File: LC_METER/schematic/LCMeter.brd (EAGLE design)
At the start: 70 x 125 mm, 212 parts, among them IC1 MEGA8535, IC10 MC34063, IC2 74HC595, IC3 74HC595, IC4 74HC595, IC5 74HC595, IC6 74HC595, IC7 LM324, IC8 7905, IC9 LM317, J10 0, J100 0, J11 0, J4 0, J6 0, J8 0, Q1 12MHz, T1 BC847, T2 BC857, T3 BC847, T4 BC847, T5 BC847, T6 BC847, T7 BC857, X1 MCU_PROGRAMMING, X2 L_X, X3 C_X, X4 USB_MICRO, X5 USB_B

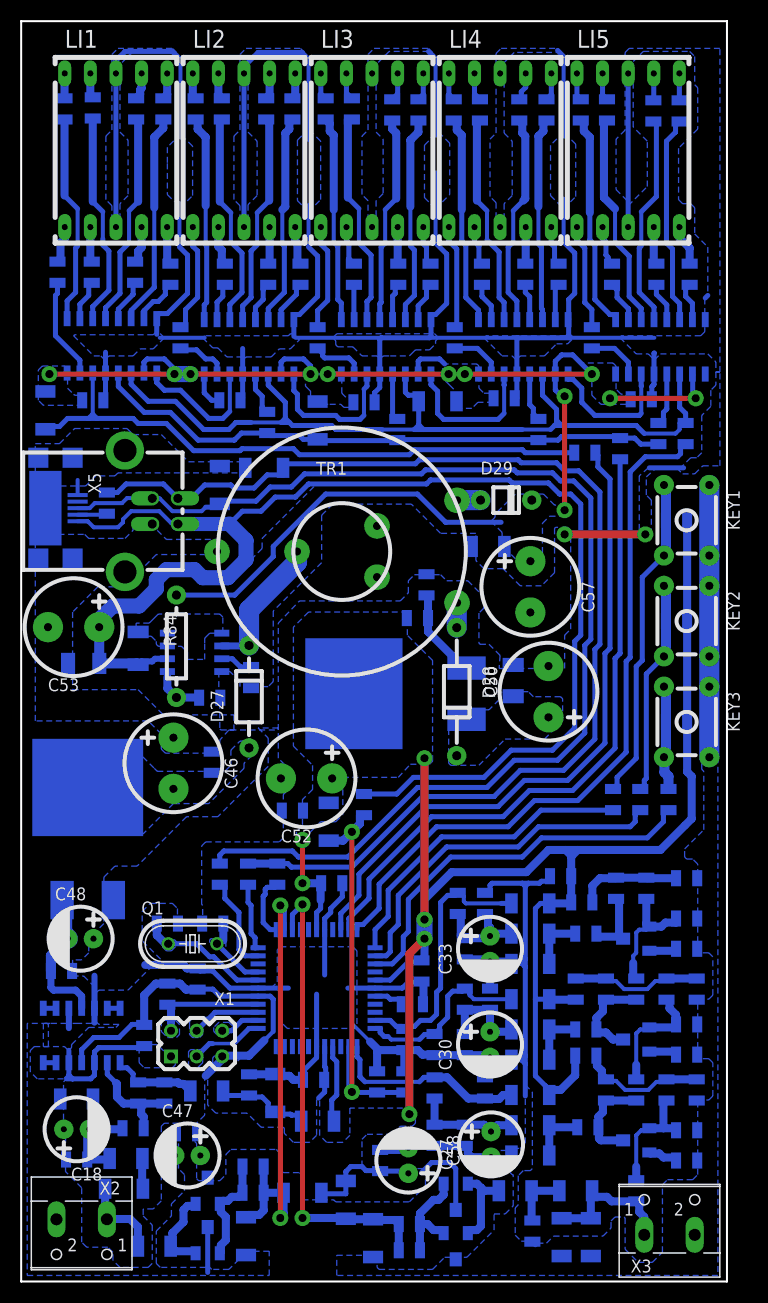
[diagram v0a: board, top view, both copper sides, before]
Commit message: LCMeter Route finished
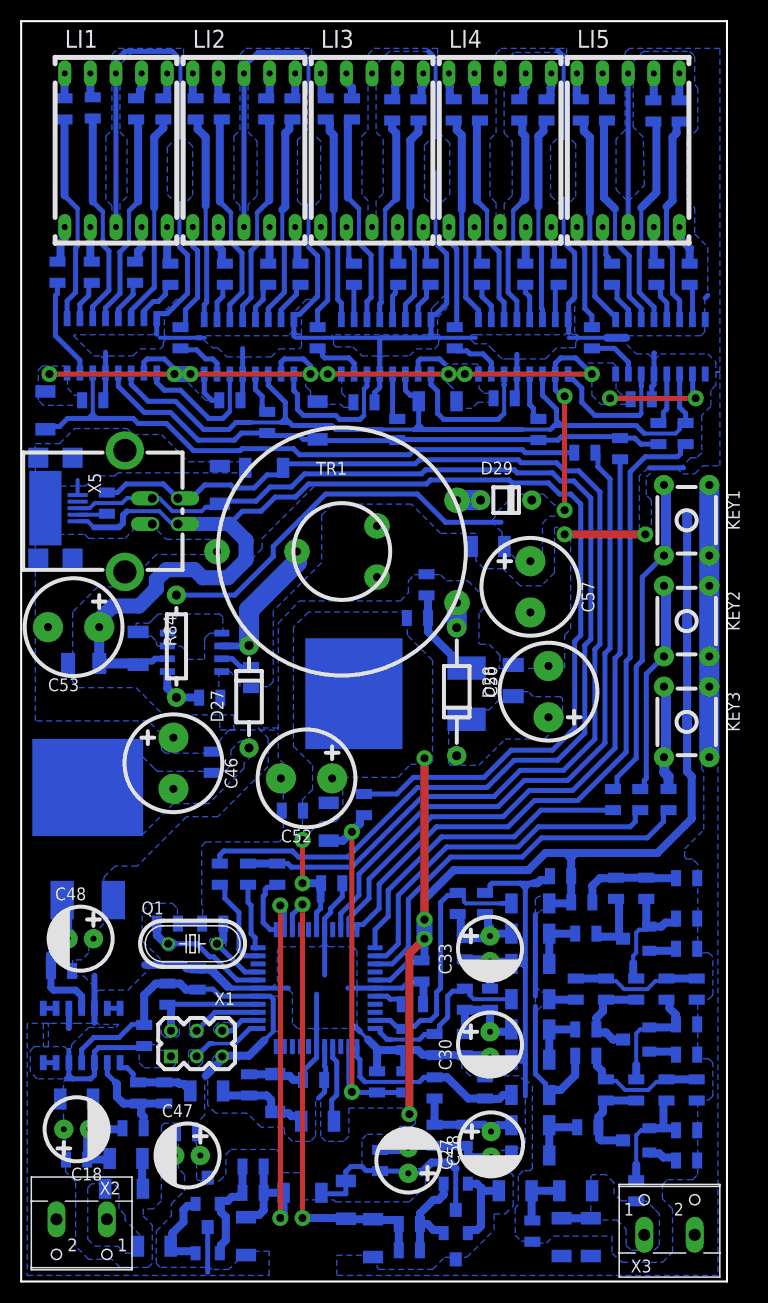
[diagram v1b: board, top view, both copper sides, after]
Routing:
- net GND: track 423.1 -> 406.6 mm
- net N$114: track 13.9 -> 2.90 mm
- net N$12: track 8.44 -> 0.00 mm
- net +5V_FINE: track 217.7 -> 212.7 mm
- net VCC_ROUGH: track 143.3 -> 141.6 mm
- net L_ADC: track 10.0 -> 9.45 mm
- added copper zone on layer 16, net N$114
- added copper zone on layer 16, net N$12

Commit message: LC meter schematic. Power stabilizer values fix
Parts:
- R81: value 5K1 -> 1K0
- R82: value 1K7 -> 3K0
- R84: value 5K1 -> 4K7
- R85: value 1K7 -> 1K6
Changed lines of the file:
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@@
 <grid distance="0.1" unitdist="mm" unit="mm" style="lines" multiple="1" display="yes" altdistance="0.025" altunitdist="inch" altunit="inch"/>
 <layers>
-<layer number="1" name="Top" color="4" fill="1" visible="no" active="yes"/>
+<layer number="1" name="Top" color="4" fill="1" visible="yes" active="yes"/>
 <layer number="2" name="Route2" color="1" fill="3" visible="no" active="no"/>
 <layer number="3" name="Route3" color="4" fill="3" visible="no" active="no"/>
@@
 <layer number="21" name="tPlace" color="7" fill="1" visible="yes" active="yes"/>
 <layer number="22" name="bPlace" color="7" fill="1" visible="yes" active="yes"/>
-<layer number="23" name="tOrigins" color="15" fill="1" visible="no" active="yes"/>
-<layer number="24" name="bOrigins" color="15" fill="1" visible="no" active="yes"/>
+<layer number="23" name="tOrigins" color="15" fill="1" visible="yes" active="yes"/>
+<layer number="24" name="bOrigins" color="15" fill="1" visible="yes" active="yes"/>
 <layer number="25" name="tNames" color="7" fill="1" visible="no" active="yes"/>
 <layer number="26" name="bNames" color="7" fill="1" visible="no" active="yes"/>
@@
 <element name="C56" library="__MyCommonLib1" package="RSMD_1206_BIG_GAP" value="0.47uFx16V" x="46.3" y="72.9" rot="MR180"/>
 <element name="C57" library="__MyCommonLib1" package="CE_10MM" value="470uFx16V" x="50.5" y="68.9" rot="R90"/>
-<element name="R84" library="__MyCommonLib1" package="R0207" value="5K1" x="15.4" y="63" rot="R90"/>
-<element name="R85" library="__MyCommonLib1" package="RSMD_0805" value="1K7" x="18.7" y="57.9" rot="MR0"/>
+<element name="R84" library="__MyCommonLib1" package="R0207" value="4K7" x="15.4" y="63" rot="R90"/>
+<element name="R85" library="__MyCommonLib1" package="RSMD_0805" value="1K6" x="18.7" y="57.9" rot="MR0"/>
 <element name="C49" library="__MyCommonLib1" package="RSMD_1206" value="0.47uFx16V" x="48.8" y="59.6" rot="MR270"/>
 <element name="C50" library="__MyCommonLib1" package="CE_10MM" value="470uFx16V" x="52.3" y="58.5" rot="R270"/>
@@
 <element name="C51" library="__MyCommonLib1" package="RSMD_0805" value="0.47uFx16V" x="26.9" y="46.7" rot="MR180"/>
 <element name="C52" library="__MyCommonLib1" package="CE_10MM" value="47uFx16V" x="28.3" y="49.9"/>
-<element name="R81" library="__MyCommonLib1" package="RSMD_0805" value="5K1" x="39.3" y="65.8" rot="MR180"/>
-<element name="R82" library="__MyCommonLib1" package="RSMD_0805" value="1K7" x="40.2" y="69.1" rot="MR270"/>
+<element name="R81" library="__MyCommonLib1" package="RSMD_0805" value="1K0" x="39.3" y="65.8" rot="MR180"/>
+<element name="R82" library="__MyCommonLib1" package="RSMD_0805" value="3K0" x="40.2" y="69.1" rot="MR270"/>
 <element name="IC8" library="__MyCommonLib1" package="D2PAK" value="7905" x="6.6" y="49" rot="MR0"/>
 <element name="C3" library="__MyCommonLib1" package="RSMD_0805" value="0.1uF" x="38.8" y="27.5" rot="MR0"/>

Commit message: LC Meter change some values
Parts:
- C47, C58: value 4.7uF -> 100uFx10V
- R54, R67, R69, R71: value 100K -> 120K
- R55, R74: value 4K7 -> 2K2
- R58: value 20K -> 24K
- R59: value 300R -> 1K0
- R75, R77, R79: value 25K -> 24K
- R86, R87, R88: value 1K0 -> 10K
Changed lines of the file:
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@@
 <layer number="49" name="Reference" color="7" fill="1" visible="no" active="yes"/>
 <layer number="51" name="tDocu" color="7" fill="1" visible="no" active="yes"/>
-<layer number="52" name="bDocu" color="7" fill="1" visible="no" active="yes"/>
+<layer number="52" name="bDocu" color="7" fill="1" visible="yes" active="yes"/>
 <layer number="91" name="Nets" color="2" fill="1" visible="no" active="no"/>
 <layer number="92" name="Busses" color="1" fill="1" visible="no" active="no"/>
@@
 <element name="R8" library="__MyCommonLib1" package="RSMD_0805" value="68R" x="25.4" y="40.4" rot="MR270"/>
 <element name="R9" library="__MyCommonLib1" package="RSMD_0805" value="1K5" x="22.5" y="40.4" rot="MR270"/>
-<element name="R55" library="__MyCommonLib1" package="RSMD_0805" value="4K7" x="23" y="11.4" rot="MR0"/>
+<element name="R55" library="__MyCommonLib1" package="RSMD_0805" value="2K2" x="23" y="11.4" rot="MR0"/>
 <element name="C17" library="__MyCommonLib1" package="RSMD_0805" value="1nF" x="23" y="8.8" rot="MR180"/>
 <element name="T1" library="__MyCommonLib1" package="SOT23_SMALL_PADS" value="BC847" x="18.5" y="9" rot="MR180"/>
@@
 <element name="C19" library="__MyCommonLib1" package="RSMD_1206_BIG_GAP" value="0.47uF" x="5.5" y="18.1" rot="MR180"/>
 <element name="R60" library="__MyCommonLib1" package="RSMD_0805" value="4K7" x="5.5" y="12.1" rot="MR0"/>
-<element name="R58" library="__MyCommonLib1" package="RSMD_0805" value="20K" x="11.1" y="15.2" rot="MR180"/>
+<element name="R58" library="__MyCommonLib1" package="RSMD_0805" value="24K" x="11.1" y="15.2" rot="MR180"/>
 <element name="C16" library="__MyCommonLib1" package="RSMD_0805" value="0.1uF" x="14.2" y="18.7" rot="MR270"/>
 <element name="IC7" library="__MyCommonLib1" package="SOIC14" value="LM324" x="6" y="24.4" rot="MR90"/>
 <element name="C25" library="__MyCommonLib1" package="RSMD_0805" value="0.1uF" x="4" y="30.8" rot="MR180"/>
 <element name="C21" library="__MyCommonLib1" package="RSMD_0805" value="0.1uF" x="12.2" y="24.4" rot="MR90"/>
-<element name="R54" library="__MyCommonLib1" package="RSMD_0805" value="100K" x="11.6" y="18.7" rot="MR90"/>
-<element name="R59" library="__MyCommonLib1" package="RSMD_1206_BIG_GAP" value="300R" x="18.4" y="18.9" rot="MR180"/>
+<element name="R54" library="__MyCommonLib1" package="RSMD_0805" value="120K" x="11.6" y="18.7" rot="MR90"/>
+<element name="R59" library="__MyCommonLib1" package="RSMD_1206_BIG_GAP" value="1K0" x="18.4" y="18.9" rot="MR180"/>
 <element name="D10" library="__MyCommonLib1" package="SOD-80" value="LL4148" x="25.2" y="18.7" rot="MR90"/>
 <element name="C20" library="__MyCommonLib1" package="RSMD_0805" value="0.1uF" x="22.6" y="19.5" rot="MR90"/>
-<element name="R74" library="__MyCommonLib1" package="RSMD_0805" value="4K7" x="38.5" y="3.1" rot="MR180"/>
+<element name="R74" library="__MyCommonLib1" package="RSMD_0805" value="2K2" x="38.5" y="3.1" rot="MR180"/>
 <element name="C39" library="__MyCommonLib1" package="RSMD_0805" value="1nF" x="38.5" y="5.7" rot="MR0"/>
 <element name="T3" library="__MyCommonLib1" package="SOT23_SMALL_PADS" value="BC847" x="43.1" y="8.4" rot="MR0"/>
@@
 <element name="T4" library="__MyCommonLib1" package="SOT23_SMALL_PADS" value="BC847" x="61" y="14" rot="MR90"/>
 <element name="C41" library="__MyCommonLib1" package="RSMD_0805" value="0.1uF" x="61" y="9" rot="MR270"/>
-<element name="R75" library="__MyCommonLib1" package="RSMD_0805" value="25K" x="66" y="15" rot="MR0"/>
-<element name="R67" library="__MyCommonLib1" package="RSMD_0805" value="100K" x="64" y="19" rot="MR90"/>
+<element name="R75" library="__MyCommonLib1" package="RSMD_0805" value="24K" x="66" y="15" rot="MR0"/>
+<element name="R67" library="__MyCommonLib1" package="RSMD_0805" value="120K" x="64" y="19" rot="MR90"/>
 <element name="R68" library="__MyCommonLib1" package="RSMD_0805" value="1K0" x="58" y="19" rot="MR90"/>
 <element name="R76" library="__MyCommonLib1" package="RSMD_0805" value="100R" x="66" y="12" rot="MR0"/>
@@
 <element name="T5" library="__MyCommonLib1" package="SOT23_SMALL_PADS" value="BC847" x="61" y="24" rot="MR90"/>
 <element name="C42" library="__MyCommonLib1" package="RSMD_0805" value="0.1uF" x="61" y="19" rot="MR270"/>
-<element name="R77" library="__MyCommonLib1" package="RSMD_0805" value="25K" x="66" y="25.5" rot="MR0"/>
-<element name="R69" library="__MyCommonLib1" package="RSMD_0805" value="100K" x="64" y="29" rot="MR90"/>
+<element name="R77" library="__MyCommonLib1" package="RSMD_0805" value="24K" x="66" y="25.5" rot="MR0"/>
+<element name="R69" library="__MyCommonLib1" package="RSMD_0805" value="120K" x="64" y="29" rot="MR90"/>
 <element name="R70" library="__MyCommonLib1" package="RSMD_0805" value="1K0" x="58" y="29" rot="MR90"/>
 <element name="R78" library="__MyCommonLib1" package="RSMD_0805" value="100R" x="66" y="22.5" rot="MR0"/>
@@
 <element name="T6" library="__MyCommonLib1" package="SOT23_SMALL_PADS" value="BC847" x="61" y="34" rot="MR90"/>
 <element name="C43" library="__MyCommonLib1" package="RSMD_0805" value="0.1uF" x="61" y="29" rot="MR270"/>
-<element name="R79" library="__MyCommonLib1" package="RSMD_0805" value="25K" x="66" y="36" rot="MR0"/>
-<element name="R71" library="__MyCommonLib1" package="RSMD_0805" value="100K" x="62" y="39" rot="MR90"/>
+<element name="R79" library="__MyCommonLib1" package="RSMD_0805" value="24K" x="66" y="36" rot="MR0"/>
+<element name="R71" library="__MyCommonLib1" package="RSMD_0805" value="120K" x="62" y="39" rot="MR90"/>
 <element name="R72" library="__MyCommonLib1" package="RSMD_0805" value="1K0" x="59" y="39" rot="MR90"/>
 <element name="R80" library="__MyCommonLib1" package="RSMD_0805" value="100R" x="66" y="33" rot="MR0"/>
@@
 <element name="X1" library="__MyCommonLib1" package="PIN2X3_2.54MM_LOOSE_PADS" value="MCU_PROGRAMMING" x="17.4" y="23.6"/>
 <element name="C48" library="__MyCommonLib1" package="CE_6.3MM" value="47uFx16V" x="5.9" y="34"/>
-<element name="R86" library="__MyCommonLib1" package="RSMD_0805" value="1K0" x="41" y="14.5" rot="MR90"/>
-<element name="R87" library="__MyCommonLib1" package="RSMD_0805" value="1K0" x="46.5" y="28" rot="MR270"/>
-<element name="R88" library="__MyCommonLib1" package="RSMD_0805" value="1K0" x="46" y="37.5" rot="MR270"/>
+<element name="R86" library="__MyCommonLib1" package="RSMD_0805" value="10K" x="41" y="14.5" rot="MR90"/>
+<element name="R87" library="__MyCommonLib1" package="RSMD_0805" value="10K" x="46.5" y="28" rot="MR270"/>
+<element name="R88" library="__MyCommonLib1" package="RSMD_0805" value="10K" x="46" y="37.5" rot="MR270"/>
 <element name="J100" library="__MyCommonLib1" package="RSMD_1206_BIG_GAP" value="0" x="29.4" y="15.9" rot="MR180"/>
-<element name="C47" library="__MyCommonLib1" package="CE_6.3MM" value="4.7uF" x="16.5" y="12.5"/>
-<element name="C58" library="__MyCommonLib1" package="CE_6.3MM" value="4.7uF" x="38.4" y="12" rot="R270"/>
+<element name="C47" library="__MyCommonLib1" package="CE_6.3MM" value="100uFx10V" x="16.5" y="12.5"/>
+<element name="C58" library="__MyCommonLib1" package="CE_6.3MM" value="100uFx10V" x="38.4" y="12" rot="R270"/>
 <element name="J11" library="__MyCommonLib1" package="RSMD_0805" value="0" x="8.5" y="77.2" rot="MR90"/>
 <element name="R100" library="__MyCommonLib1" package="RSMD_0805" value="10K" x="34" y="47.3" rot="MR270"/>

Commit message: LC Meter. Battery voltage metter resistors values changed
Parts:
- R89: value 1K -> 3K0
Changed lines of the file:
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@@
 <element name="J11" library="__MyCommonLib1" package="RSMD_0805" value="0" x="8.5" y="77.2" rot="MR90"/>
 <element name="R100" library="__MyCommonLib1" package="RSMD_0805" value="10K" x="34" y="47.3" rot="MR270"/>
-<element name="R89" library="__MyCommonLib1" package="RSMD_0805" value="1K" x="35.3" y="19.8" rot="MR90"/>
+<element name="R89" library="__MyCommonLib1" package="RSMD_0805" value="3K0" x="35.3" y="19.8" rot="MR90"/>
 <element name="C4" library="__MyCommonLib1" package="RSMD_0805" value="0.1uF" x="38" y="19.8" rot="MR270"/>
 <element name="D4" library="__MyCommonLib1" package="SOD-80" value="LL4148" x="30.5" y="45.6" rot="MR270"/>
